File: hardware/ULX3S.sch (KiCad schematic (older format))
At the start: 2 parts

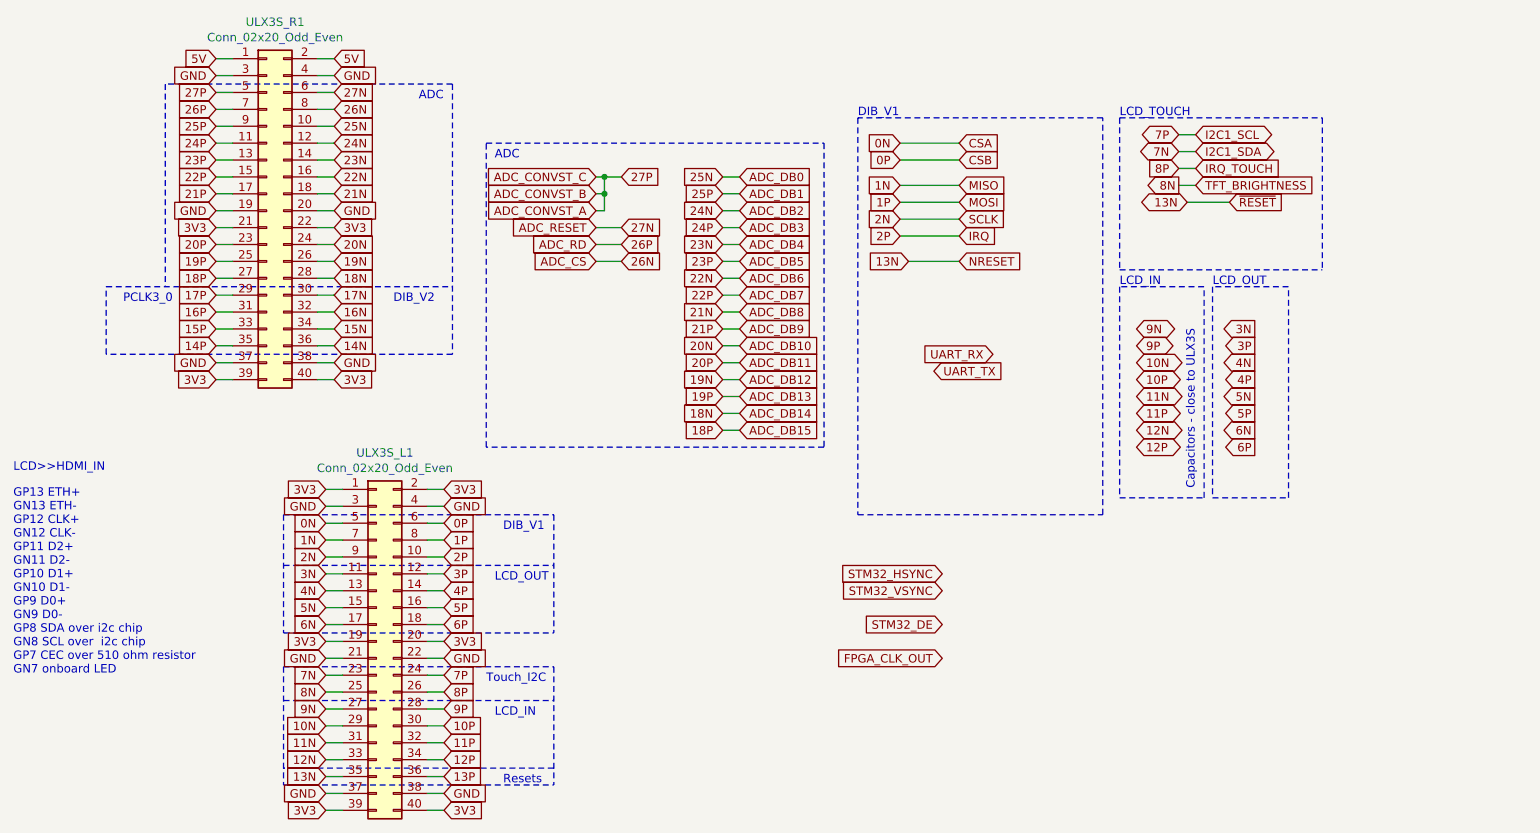
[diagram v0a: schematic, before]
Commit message: Adding last known changes to shematics
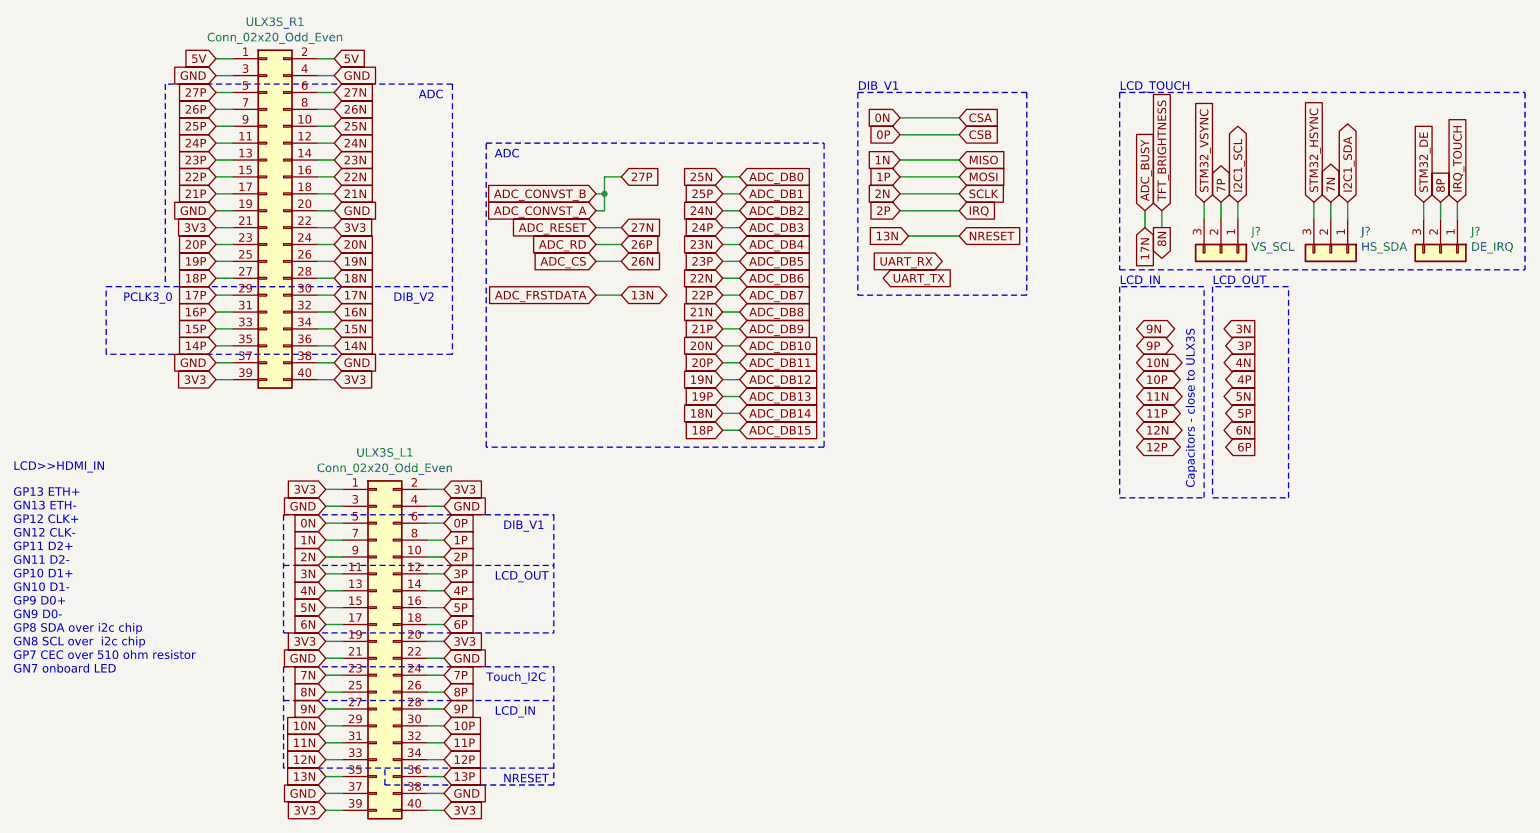
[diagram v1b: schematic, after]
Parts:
- added J?: VS_SCL, symbol Connector_Generic:Conn_01x03
- added J?: DE_IRQ, symbol Connector_Generic:Conn_01x03
- added J?: HS_SDA, symbol Connector_Generic:Conn_01x03
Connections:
- net 7N: now also J?.2 (Pin_2)
- net 7P: now also J?.2 (Pin_2)
- net 8P: now also J?.2 (Pin_2)
- net STM32_DE: now also J?.3 (Pin_3)
- net STM32_HSYNC: now also J?.3 (Pin_3)
- net STM32_VSYNC: now also J?.3 (Pin_3)
- new net I2C1_SCL: J?.1 (Pin_1)
- new net I2C1_SDA: J?.1 (Pin_1)
- new net IRQ_TOUCH: J?.1 (Pin_1)
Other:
- note added: "NRESET"
- note removed: "Resets"
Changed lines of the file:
@@
 $Descr A4 11693 8268
 encoding utf-8
-Sheet 3 11
+Sheet 3 10
 Title ""
-Date ""
-Rev ""
-Comp ""
+Date "2020-01-29"
+Rev "0.1"
+Comp "Envox d.o.o."
 Comment1 ""
 Comment2 ""
@@
 Text Notes 750  3450 0    50   ~ 0
 LCD>>HDMI_IN
-Text GLabel 6350 1750 2    50   Input ~ 0
+Text GLabel 6350 1600 2    50   Input ~ 0
 MISO
-Text GLabel 6350 1500 2    50   Input ~ 0
+Text GLabel 6350 1350 2    50   Input ~ 0
 CSA
-Text GLabel 6350 1600 2    50   Input ~ 0
+Text GLabel 6350 1450 2    50   Input ~ 0
 CSB
-Text GLabel 6350 1850 2    50   Input ~ 0
+Text GLabel 6350 1700 2    50   Input ~ 0
 MOSI
-Text GLabel 6350 1950 2    50   Input ~ 0
+Text GLabel 6350 1800 2    50   Input ~ 0
 SCLK
-Text GLabel 6350 2050 2    50   Input ~ 0
+Text GLabel 6350 1900 2    50   Input ~ 0
 IRQ
-Text GLabel 6350 2200 2    50   Input ~ 0
+Text GLabel 6350 2050 2    50   Input ~ 0
 NRESET
-Text GLabel 6550 2750 0    50   Input ~ 0
+Text GLabel 6250 2200 0    50   Input ~ 0
 UART_RX
-Text GLabel 6200 2850 2    50   Input ~ 0
+Text GLabel 5900 2300 2    50   Input ~ 0
 UART_TX
-Wire Notes Line
-	5750 3700 7200 3700
-Wire Notes Line
-	7200 3700 7200 1350
-Wire Notes Line
-	7200 1350 5750 1350
-Wire Notes Line
-	5750 1350 5750 3700
-Text Notes 5750 1350 0    50   ~ 0
+Text Notes 5750 1200 0    50   ~ 0
 DIB_V1
-Text GLabel 7650 1450 0    50   BiDi ~ 0
-7P
-Text GLabel 7650 1550 0    50   BiDi ~ 0
-7N
-Text GLabel 7750 1450 2    50   BiDi ~ 0
-I2C1_SCL
-Text GLabel 7750 1550 2    50   BiDi ~ 0
-I2C1_SDA
-Wire Wire Line
-	7650 1450 7750 1450
-Wire Wire Line
-	7650 1550 7750 1550
-Text GLabel 7650 1650 0    50   Input ~ 0
+Text GLabel 9200 1850 1    50   Input ~ 0
 8P
-Wire Wire Line
-	7650 1650 7750 1650
-Text GLabel 7650 1750 0    50   Output ~ 0
+Text GLabel 7550 2000 3    50   Output ~ 0
 8N
 Wire Wire Line
-	7650 1750 7750 1750
-Text GLabel 7950 1850 2    50   Input ~ 0
-~RESET
-Text GLabel 7750 1650 2    50   Input ~ 0
+	7550 2000 7550 1900
+Text GLabel 9300 1850 1    50   Input ~ 0
 IRQ_TOUCH
-Text GLabel 7750 1750 2    50   Input ~ 0
+Text GLabel 7550 1900 1    50   Input ~ 0
 TFT_BRIGHTNESS
-Text GLabel 7700 1850 0    50   BiDi ~ 0
+Text GLabel 4350 2400 2    50   BiDi ~ 0
 13N
-Wire Notes Line
-	7300 1350 8500 1350
-Wire Notes Line
-	8500 1350 8500 2250
-Wire Notes Line
-	7300 1350 7300 2250
-Wire Notes Line
-	7300 2250 8500 2250
-Text Notes 7300 1350 0    50   ~ 0
+Text Notes 7300 1200 0    50   ~ 0
 LCD_TOUCH
-Wire Wire Line
-	7950 1850 7700 1850
 Text GLabel 7400 3300 2    50   BiDi ~ 0
 12P
@@
 Text Notes 3650 3800 0    50   ~ 0
 DIB_V1
-Text GLabel 6000 1500 0    50   Input ~ 0
+Text GLabel 6000 1350 0    50   Input ~ 0
 0N
-Text GLabel 6000 1750 0    50   Input ~ 0
+Text GLabel 6000 1600 0    50   Input ~ 0
 1N
-Text GLabel 6000 1950 0    50   Input ~ 0
+Text GLabel 6000 1800 0    50   Input ~ 0
 2N
-Text GLabel 6000 1600 0    50   Input ~ 0
+Text GLabel 6000 1450 0    50   Input ~ 0
 0P
-Text GLabel 6000 1850 0    50   Input ~ 0
+Text GLabel 6000 1700 0    50   Input ~ 0
 1P
-Text GLabel 6000 2050 0    50   Input ~ 0
+Text GLabel 6000 1900 0    50   Input ~ 0
 2P
-Text GLabel 6050 2200 0    50   Input ~ 0
+Text GLabel 6050 2050 0    50   Input ~ 0
 13N
 Wire Wire Line
-	6000 1500 6350 1500
+	6000 1350 6350 1350
 Wire Wire Line
-	6000 1600 6350 1600
+	6000 1450 6350 1450
 Wire Wire Line
-	6000 1750 6350 1750
+	6000 1600 6350 1600
 Wire Wire Line
-	6000 1850 6350 1850
+	6000 1700 6350 1700
 Wire Wire Line
-	6000 1950 6350 1950
+	6000 1800 6350 1800
 Wire Wire Line
-	6050 2200 6350 2200
+	6050 2050 6350 2050
 Wire Wire Line
-	6000 2050 6350 2050
-Wire Notes Line
-	2350 5300 3950 5300
-Wire Notes Line
-	2350 4600 2350 5300
+	6000 1900 6350 1900
 Wire Notes Line
 	3950 4600 3950 5300
 Text Notes 3650 5300 0    50   ~ 0
-Resets
+NRESET
 Wire Wire Line
 	4950 1700 5050 1700
@@
 Text GLabel 4200 1800 0    50   Input ~ 0
 ADC_CONVST_B
-Text GLabel 4200 1700 0    50   Input ~ 0
-ADC_CONVST_C
 Text GLabel 4200 2100 0    50   Input ~ 0
 ADC_RD
@@
 22N
 Wire Wire Line
-	4200 1700 4250 1700
-Wire Wire Line
 	4200 1800 4250 1800
 Wire Wire Line
 	4250 1800 4250 1700
-Connection ~ 4250 1700
 Wire Wire Line
 	4250 1700 4350 1700
@@
 Text Notes 3000 2450 0    50   ~ 0
 DIB_V2
-Text GLabel 6250 4050 0    50   Input ~ 0
+Text GLabel 8450 1850 1    50   Input ~ 0
 STM32_HSYNC
-Text GLabel 6250 4150 0    50   Input ~ 0
+Text GLabel 7800 1850 1    50   Input ~ 0
 STM32_VSYNC
-Text GLabel 6250 4350 0    50   Input ~ 0
+Text GLabel 9100 1850 1    50   Input ~ 0
 STM32_DE
-Text GLabel 6250 4550 0    50   Input ~ 0
-FPGA_CLK_OUT
+Text GLabel 7450 1900 1    50   Input ~ 0
+ADC_BUSY
+Text GLabel 4200 2400 0    50   Input ~ 0
+ADC_FRSTDATA
+Wire Wire Line
+	4200 2400 4350 2400
+Wire Notes Line
+	2350 4600 2350 5200
+Wire Notes Line
+	3950 5300 2950 5300
+Wire Notes Line
+	2950 5300 2950 5200
+$Comp
+L Connector_Generic:Conn_01x03 J?
+U 1 1 5E7481BA
+P 7900 2150
+AR Path="/5E22D897/5E776450/5E7481BA" Ref="J?"  Part="1"
+AR Path="/5E22C01C/5E7481BA" Ref="J?"  Part="1"
+F 0 "J?" V 7773 2330 50  0000 L CNN
+F 1 "VS_SCL" V 7864 2330 50  0000 L CNN
+F 2 "" H 7900 2150 50  0001 C CNN
+F 3 "~" H 7900 2150 50  0001 C CNN
+	1    7900 2150
+	0    1    1    0
+$EndComp
+Text GLabel 8000 1850 1    50   BiDi ~ 0
+I2C1_SCL
+Text GLabel 7900 1850 1    50   BiDi ~ 0
+7P
+$Comp
+L Connector_Generic:Conn_01x03 J?
+U 1 1 5E7548B6
+P 9200 2150
+AR Path="/5E22D897/5E776450/5E7548B6" Ref="J?"  Part="1"
+AR Path="/5E22C01C/5E7548B6" Ref="J?"  Part="1"
+F 0 "J?" V 9073 2330 50  0000 L CNN
+F 1 "DE_IRQ" V 9164 2330 50  0000 L CNN
+F 2 "" H 9200 2150 50  0001 C CNN
+F 3 "~" H 9200 2150 50  0001 C CNN
+	1    9200 2150
+	0    1    1    0
+$EndComp
+Text GLabel 8650 1850 1    50   BiDi ~ 0
+I2C1_SDA
+Text GLabel 8550 1850 1    50   BiDi ~ 0
+7N
+$Comp
+L Connector_Generic:Conn_01x03 J?
+U 1 1 5E772205
+P 8550 2150
+AR Path="/5E22D897/5E776450/5E772205" Ref="J?"  Part="1"
+AR Path="/5E22C01C/5E772205" Ref="J?"  Part="1"
+F 0 "J?" V 8423 2330 50  0000 L CNN
+F 1 "HS_SDA" V 8514 2330 50  0000 L CNN
+F 2 "" H 8550 2150 50  0001 C CNN
+F 3 "~" H 8550 2150 50  0001 C CNN
+	1    8550 2150
+	0    1    1    0
+$EndComp
+Text GLabel 7450 2000 3    50   Input ~ 0
+17N
+Wire Wire Line
+	7450 2000 7450 1900
+Wire Wire Line
+	9300 1850 9300 1950
+Wire Wire Line
+	9200 1850 9200 1950
+Wire Wire Line
+	9100 1850 9100 1950
+Wire Wire Line
+	8650 1850 8650 1950
+Wire Wire Line
+	8550 1850 8550 1950
+Wire Wire Line
+	8450 1850 8450 1950
+Wire Wire Line
+	8000 1850 8000 1950
+Wire Wire Line
+	7900 1850 7900 1950
+Wire Wire Line
+	7800 1850 7800 1950
+Wire Notes Line
+	7300 1200 9700 1200
+Wire Notes Line
+	9700 1200 9700 2250
+Wire Notes Line
+	7300 1200 7300 2250
+Wire Notes Line
+	7300 2250 9700 2250
+Wire Notes Line
+	5750 1200 5750 2400
+Wire Notes Line
+	5750 1200 6750 1200
+Wire Notes Line
+	6750 1200 6750 2400
+Wire Notes Line
+	6750 2400 5750 2400
 $EndSCHEMATC
